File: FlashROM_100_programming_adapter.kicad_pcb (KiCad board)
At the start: 2 copper layers, 16.8 x 39.6 mm, 3 parts, among them J1 LH535618 Socket, U1 29F010 pins to programmer

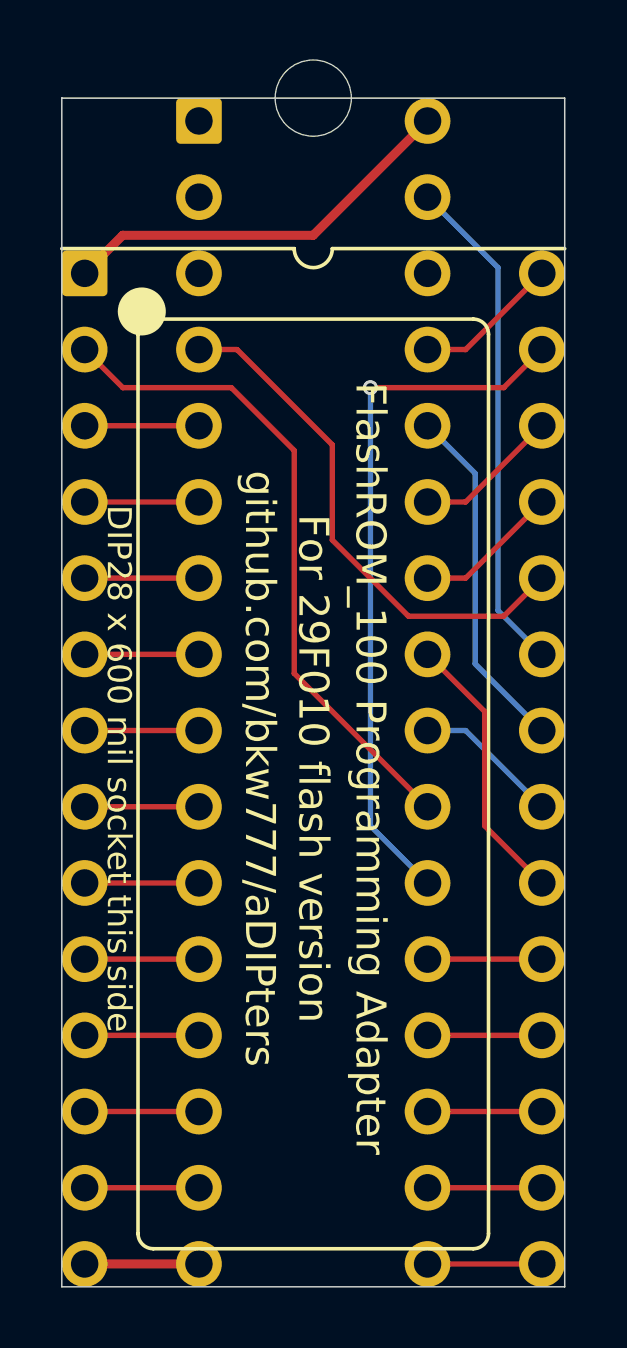
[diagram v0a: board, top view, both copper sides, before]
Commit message: kicad 6
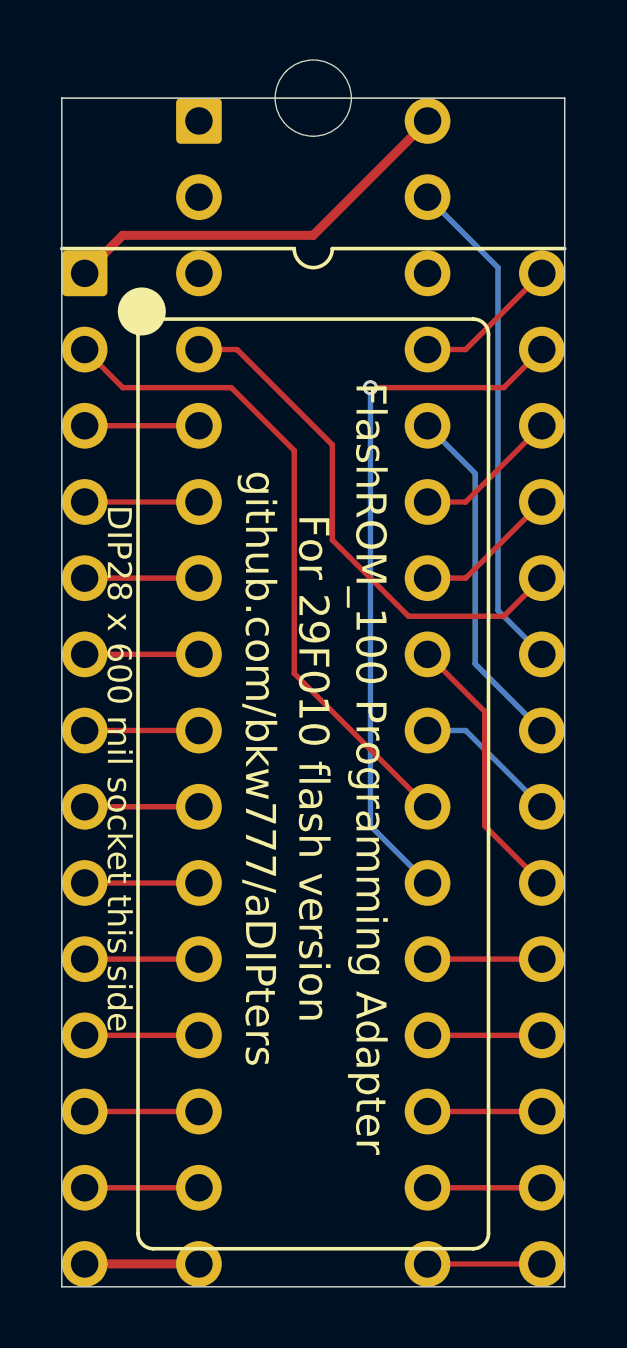
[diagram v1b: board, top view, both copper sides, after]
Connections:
- net /~CE renamed /~{CE}
- net /~OE renamed /~{OE}
- net /~WE renamed /~{WE}
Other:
- net class Default removed
